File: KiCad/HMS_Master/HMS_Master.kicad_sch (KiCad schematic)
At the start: 5 parts, among them J1 JST 2P, U1 ESP32-DEVKITC-32UE

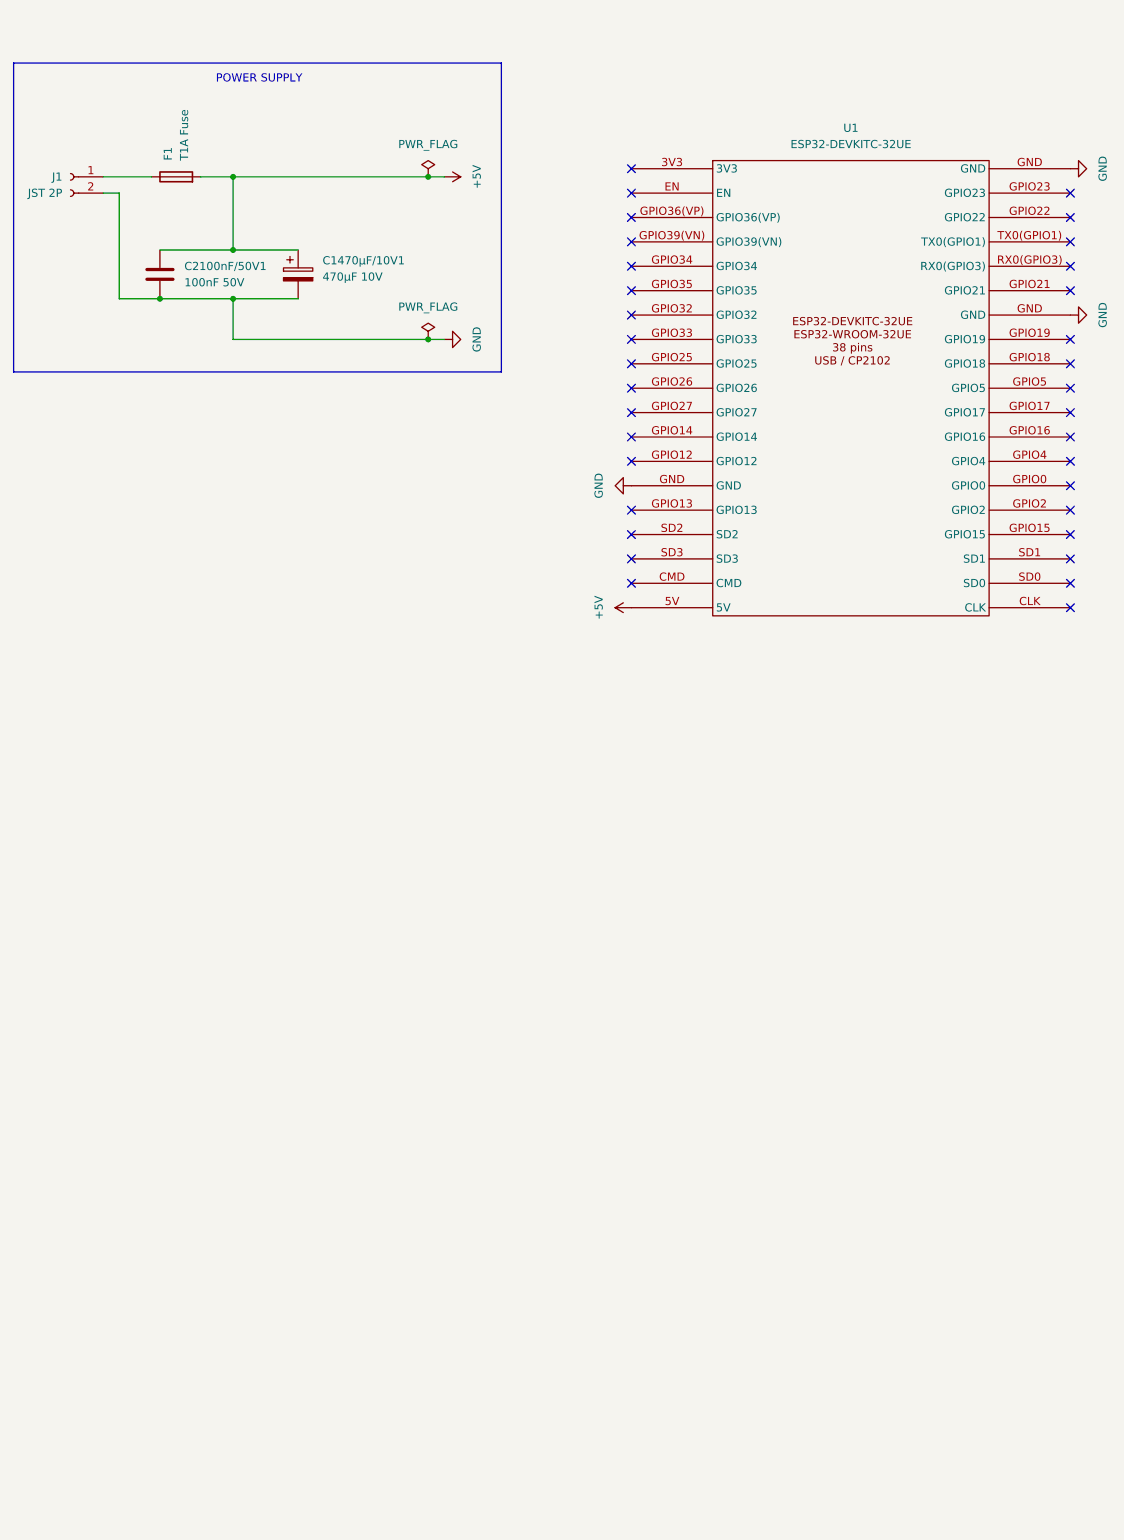
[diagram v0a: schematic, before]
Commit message: Schematic Complete
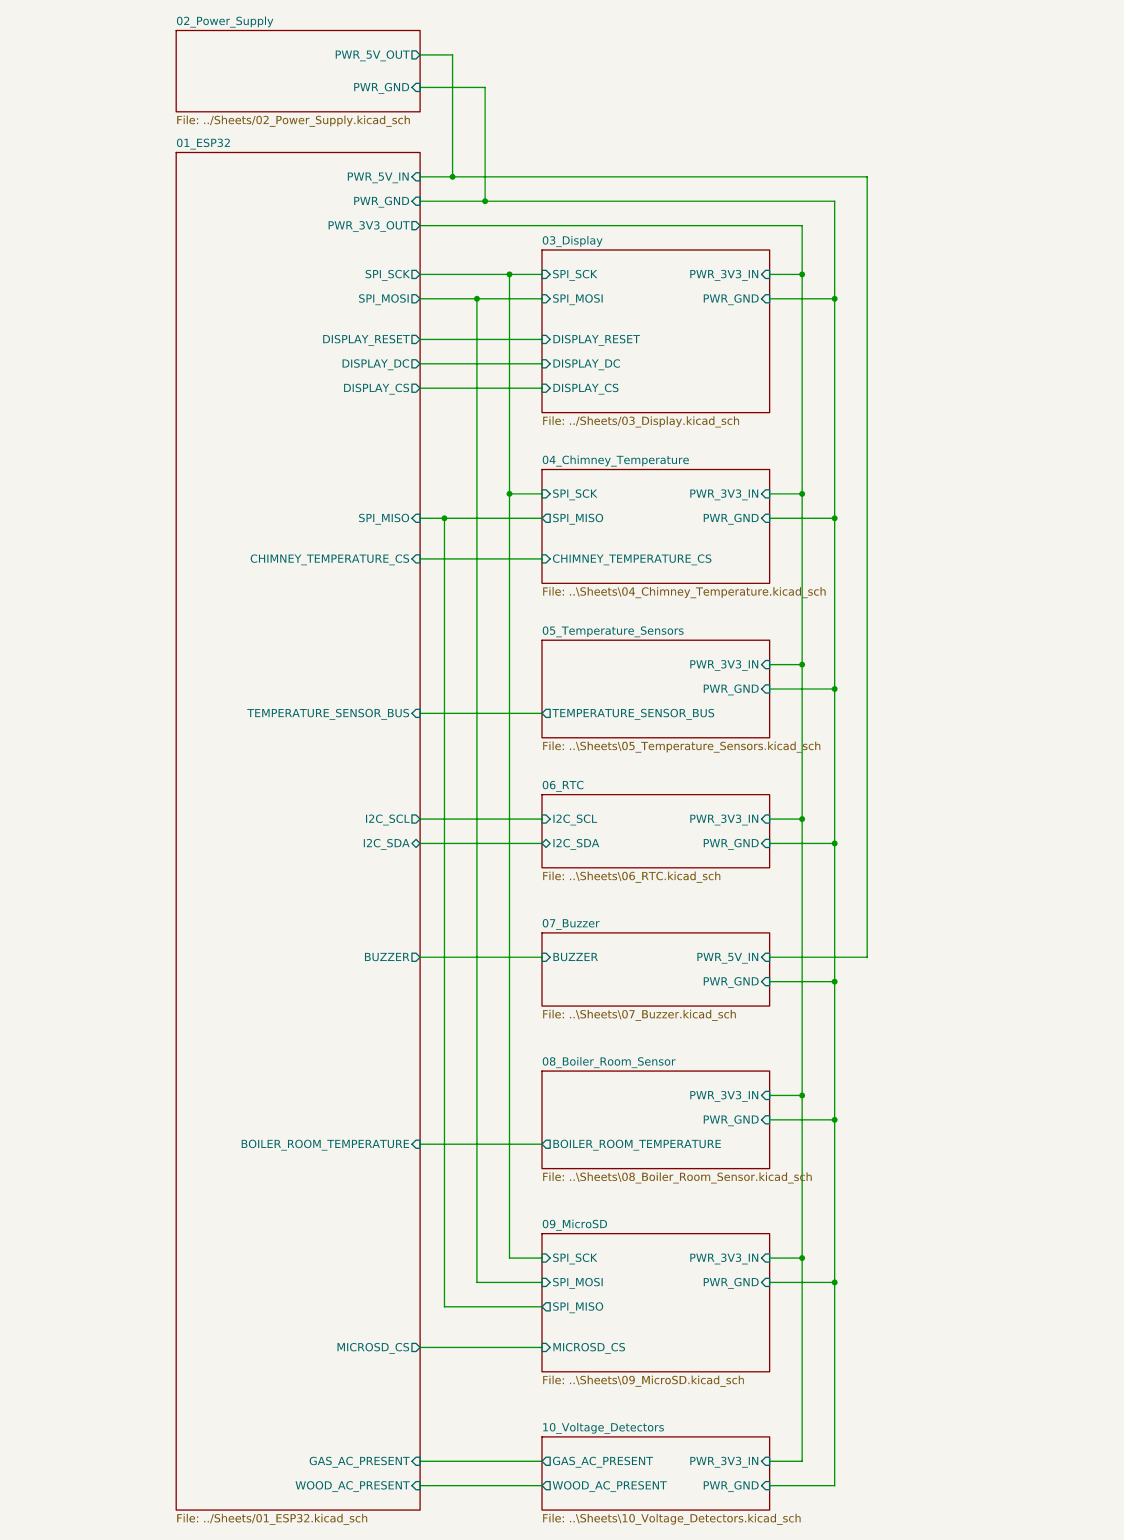
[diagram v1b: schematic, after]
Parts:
- removed C1470µF/10V1: 470µF 10V, symbol Device:C_Polarized
- removed C2100nF/50V1: 100nF 50V, symbol Device:C
- removed F1: T1A Fuse, symbol Device:Fuse
- removed J1: JST 2P, symbol Connector:Conn_01x02_Socket
- removed U1: ESP32-DEVKITC-32UE, symbol HMS_Symbols:ESP32_DEVKITC_32UE
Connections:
- no-connect marks 34 -> 0
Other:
- added sheet 01_ESP32 (../Sheets/01_ESP32.kicad_sch)
- added sheet 02_Power_Supply (../Sheets/02_Power_Supply.kicad_sch)
- added sheet 03_Display (../Sheets/03_Display.kicad_sch)
- added sheet 04_Chimney_Temperature (..\Sheets\04_Chimney_Temperature.kicad_sch)
- added sheet 05_Temperature_Sensors (..\Sheets\05_Temperature_Sensors.kicad_sch)
- added sheet 06_RTC (..\Sheets\06_RTC.kicad_sch)
- added sheet 07_Buzzer (..\Sheets\07_Buzzer.kicad_sch)
- added sheet 08_Boiler_Room_Sensor (..\Sheets\08_Boiler_Room_Sensor.kicad_sch)
- added sheet 09_MicroSD (..\Sheets\09_MicroSD.kicad_sch)
- added sheet 10_Voltage_Detectors (..\Sheets\10_Voltage_Detectors.kicad_sch)
- note removed: "POWER SUPPLY"
